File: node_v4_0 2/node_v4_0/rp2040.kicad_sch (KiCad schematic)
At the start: 29 parts, among them U1 RP2040, U2 W25Q128JVS, U7 PTS526 SK15 SMTR2 LFS, U8 PTS526 SK15 SMTR2 LFS

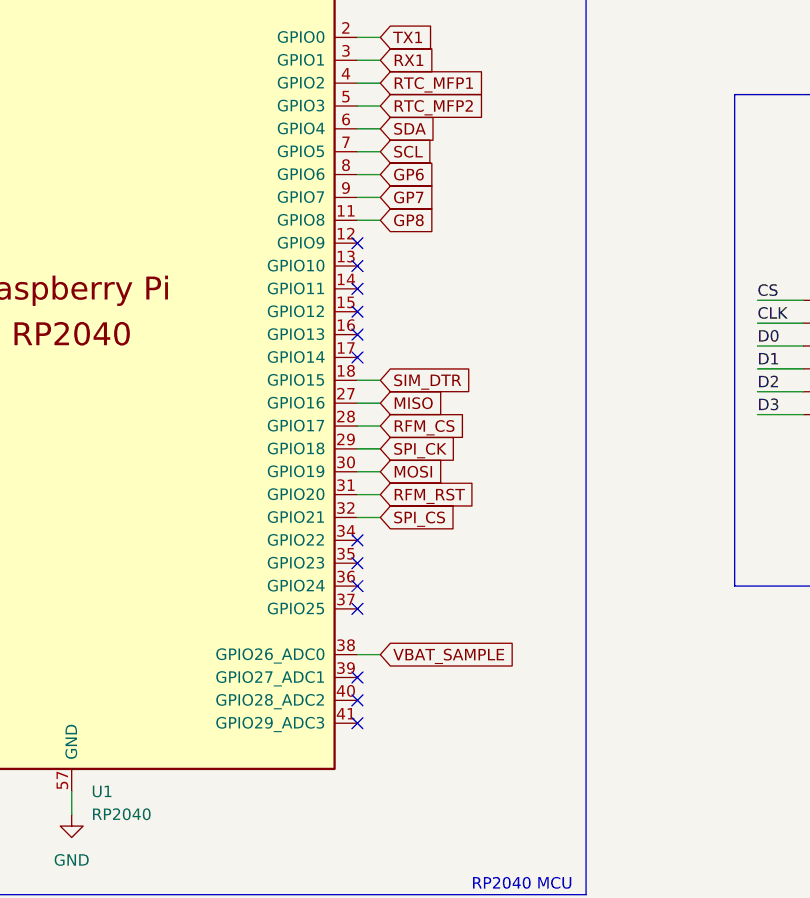
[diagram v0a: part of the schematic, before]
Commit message: most routing done
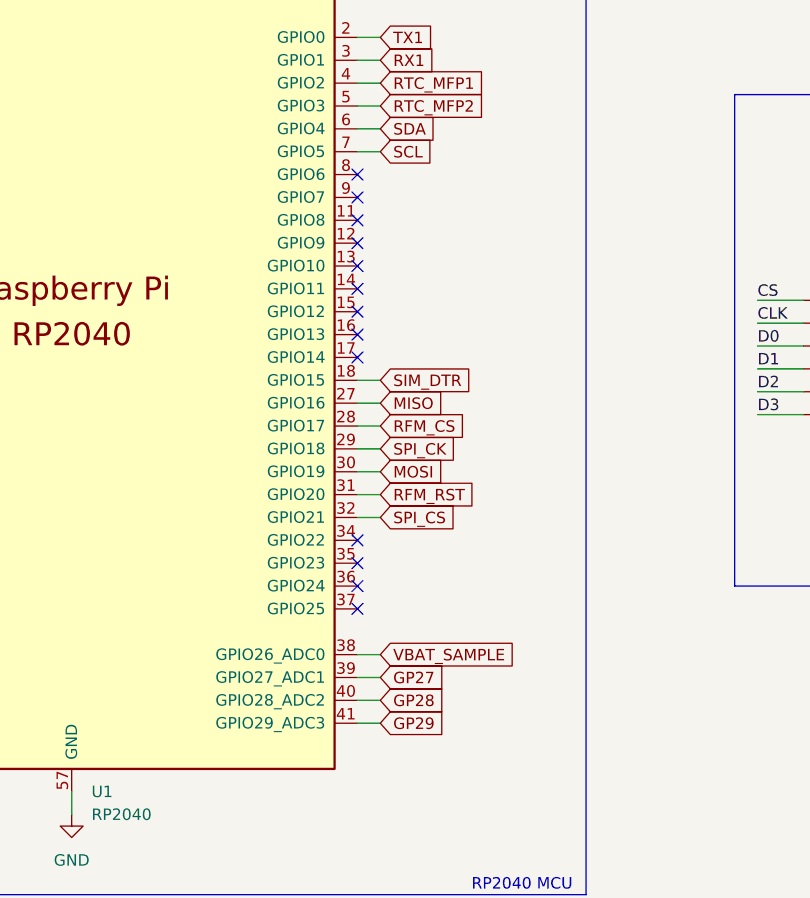
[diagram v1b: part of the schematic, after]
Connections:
- net GP27: now reaches U1.39 (GPIO27_ADC1)
- net GP28: now reaches U1.40 (GPIO28_ADC2)
- net GP29: now reaches U1.41 (GPIO29_ADC3)
- net GP6: no longer names the net of U1.8 (GPIO6)
- net GP7: no longer names the net of U1.9 (GPIO7)
- net GP8: no longer names the net of U1.11 (GPIO8)
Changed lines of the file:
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@@
+	)
+	(no_connect
+		(at 95.25 120.65)
+	)
+	(no_connect
+		(at 95.25 115.57)
 	)
 	(no_connect
@@
 	)
 	(no_connect
-		(at 95.25 173.99)
-	)
-	(no_connect
 		(at 95.25 128.27)
 	)
@@
 	)
 	(no_connect
-		(at 95.25 176.53)
+		(at 95.25 118.11)
 	)
 	(no_connect
@@
 		(at 95.25 123.19)
 	)
-	(no_connect
-		(at 95.25 171.45)
-	)
 	(wire
 		(pts
@@
 	(wire
 		(pts
-			(xy 95.25 115.57) (xy 97.79 115.57)
-		)
-		(stroke
-			(width 0)
-			(type default)
-		)
-	)
-	(wire
-		(pts
 			(xy 59.69 76.2) (xy 59.69 82.55)
 		)
@@
 	(wire
 		(pts
-			(xy 95.25 120.65) (xy 97.79 120.65)
-		)
-		(stroke
-			(width 0)
-			(type default)
-		)
-	)
-	(wire
-		(pts
 			(xy 95.25 107.95) (xy 97.79 107.95)
 		)
@@
 	(wire
 		(pts
-			(xy 95.25 118.11) (xy 97.79 118.11)
-		)
-		(stroke
-			(width 0)
-			(type default)
-		)
-	)
-	(wire
-		(pts
 			(xy 173.99 127) (xy 173.99 128.27)
 		)
@@
 	(wire
 		(pts
+			(xy 95.25 176.53) (xy 97.79 176.53)
+		)
+		(stroke
+			(width 0)
+			(type default)
+		)
+	)
+	(wire
+		(pts
 			(xy 173.99 118.11) (xy 186.69 118.11)
 		)
@@
 	(wire
 		(pts
+			(xy 95.25 171.45) (xy 97.79 171.45)
+		)
+		(stroke
+			(width 0)
+			(type default)
+		)
+	)
+	(wire
+		(pts
 			(xy 80.01 76.2) (xy 80.01 82.55)
 		)
@@
 		(pts
 			(xy 233.68 33.02) (xy 233.68 31.75)
+		)
+		(stroke
+			(width 0)
+			(type default)
+		)
+	)
+	(wire
+		(pts
+			(xy 95.25 173.99) (xy 97.79 173.99)
 		)
 		(stroke
@@
 		)
 	)
-	(global_label "GP8"
-		(shape input)
-		(at 97.79 120.65 0)
-		(fields_autoplaced yes)
-		(effects
-			(font
-				(size 1.27 1.27)
-			)
-			(justify left)
-		)
-		(property "Intersheetrefs" "${INTERSHEET_REFS}"
-			(at 104.5247 120.65 0)
-			(effects
-				(font
-					(size 1.27 1.27)
-				)
-				(justify left)
-				(hide yes)
-			)
-		)
-	)
 	(global_label "SDA"
 		(shape input)
@@
 		)
 	)
-	(global_label "GP7"
-		(shape input)
-		(at 97.79 118.11 0)
-		(fields_autoplaced yes)
-		(effects
-			(font
-				(size 1.27 1.27)
-			)
-			(justify left)
-		)
-		(property "Intersheetrefs" "${INTERSHEET_REFS}"
-			(at 104.5247 118.11 0)
-			(effects
-				(font
-					(size 1.27 1.27)
-				)
-				(justify left)
-				(hide yes)
-			)
-		)
-	)
 	(global_label "TX1"
 		(shape input)
@@
 		)
 	)
-	(global_label "GP6"
-		(shape input)
-		(at 97.79 115.57 0)
-		(fields_autoplaced yes)
-		(effects
-			(font
-				(size 1.27 1.27)
-			)
-			(justify left)
-		)
-		(property "Intersheetrefs" "${INTERSHEET_REFS}"
-			(at 104.5247 115.57 0)
-			(effects
-				(font
-					(size 1.27 1.27)
-				)
-				(justify left)
-				(hide yes)
-			)
-		)
-	)
 	(global_label "SWCLK"
 		(shape input)
@@
 		)
 	)
+	(global_label "GP28"
+		(shape input)
+		(at 97.79 173.99 0)
+		(fields_autoplaced yes)
+		(effects
+			(font
+				(size 1.27 1.27)
+			)
+			(justify left)
+		)
+		(property "Intersheetrefs" "${INTERSHEET_REFS}"
+			(at 105.7342 173.99 0)
+			(effects
+				(font
+					(size 1.27 1.27)
+				)
+				(justify left)
+				(hide yes)
+			)
+		)
+	)
 	(global_label "RFM_CS"
 		(shape input)
@@
 		)
 	)
+	(global_label "GP29"
+		(shape input)
+		(at 97.79 176.53 0)
+		(fields_autoplaced yes)
+		(effects
+			(font
+				(size 1.27 1.27)
+			)
+			(justify left)
+		)
+		(property "Intersheetrefs" "${INTERSHEET_REFS}"
+			(at 105.7342 176.53 0)
+			(effects
+				(font
+					(size 1.27 1.27)
+				)
+				(justify left)
+				(hide yes)
+			)
+		)
+	)
 	(global_label "VBAT_SAMPLE"
 		(shape input)
@@
 			(effects
 				(font
+					(size 1.27 1.27)
+				)
+				(justify left)
+				(hide yes)
+			)
+		)
+	)
+	(global_label "GP27"
+		(shape input)
+		(at 97.79 171.45 0)
+		(fields_autoplaced yes)
+		(effects
+			(font
+				(size 1.27 1.27)
+			)
+			(justify left)
+		)
+		(property "Intersheetrefs" "${INTERSHEET_REFS}"
+			(at 105.7342 171.45 0)
+			(effects
+				(font
